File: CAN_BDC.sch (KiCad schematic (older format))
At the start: 24 parts, among them P1 CONN_01X05, P2 CONN_01X02, P3 CONN_01X02, P5 CONN_01X02, U1 STM32F042C6Ux, U2 PSD2CAN, U3 SN65HVD232D, U4 drv8850, U5 MCP1700T-3302E/TT

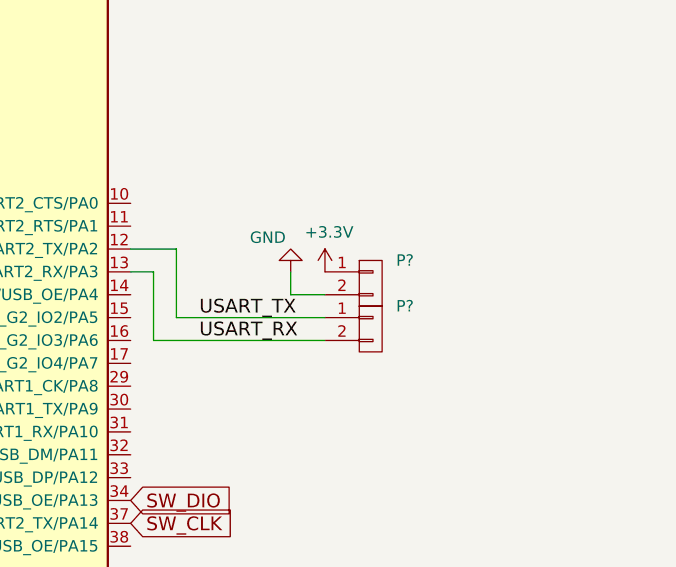
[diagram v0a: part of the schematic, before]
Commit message: Connector update
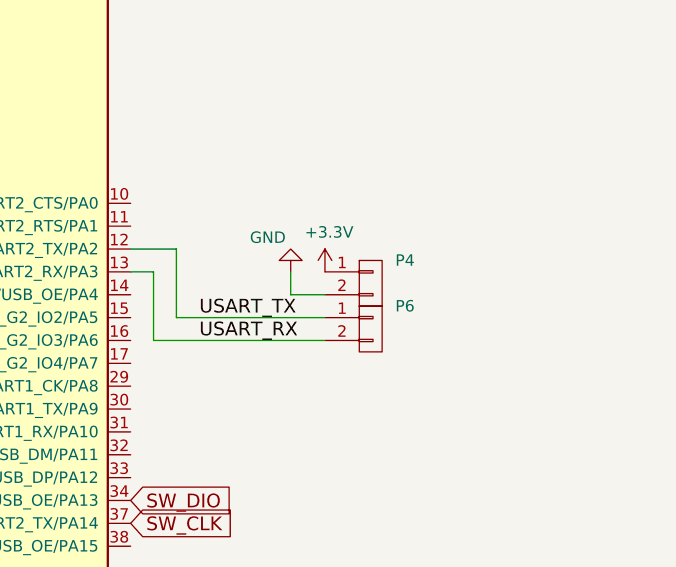
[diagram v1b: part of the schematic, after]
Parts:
- gave numbers to parts that had none: 2
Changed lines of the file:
@@
 	1550 1350 1250 1350
 $Comp
-L GND #PWR02
+L GND #PWR030
 U 1 1 57056C83
 P 1550 1350
-F 0 "#PWR02" H 1550 1100 50  0001 C CNN
+F 0 "#PWR030" H 1550 1100 50  0001 C CNN
 F 1 "GND" V 1558 1222 50  0000 R CNN
 F 2 "" H 1550 1350 50  0000 C CNN
@@
 $EndComp
 $Comp
-L CONN_01X02 P?
+L CONN_01X02 P4
 U 1 1 57FD66CE
 P 9700 2900
-F 0 "P?" H 9850 3000 50  0000 C CNN
+F 0 "P4" H 9850 3000 50  0000 C CNN
 F 1 "CONN_01X02" V 9574 2756 50  0001 R CNN
 F 2 "Pin_Headers:Pin_Header_Straight_1x02" H 9700 2900 50  0001 C CNN
@@
 $EndComp
 $Comp
-L CONN_01X02 P?
+L CONN_01X02 P6
 U 1 1 57FD69A3
 P 9700 3100
-F 0 "P?" H 9850 3200 50  0000 C CNN
+F 0 "P6" H 9850 3200 50  0000 C CNN
 F 1 "CONN_01X02" V 9574 2956 50  0001 R CNN
 F 2 "Pin_Headers:Pin_Header_Straight_1x02" H 9700 3100 50  0001 C CNN
